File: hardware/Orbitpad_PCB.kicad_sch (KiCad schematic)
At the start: 50 parts, among them J1 Conn_01x04_Pin, SW1 SW_Push, SW10 SW_Push, SW11 SW_Push, SW12 SW_Push, SW13 SW_Push, SW14 SW_Push, SW15 SW_Push, SW16 SW_Push, SW2 SW_Push, SW3 SW_Push, SW4 SW_Push, SW5 SW_Push, SW6 SW_Push, SW7 SW_Push, SW8 SW_Push, SW9 SW_Push, U1 XIAO-RP2040-DIP

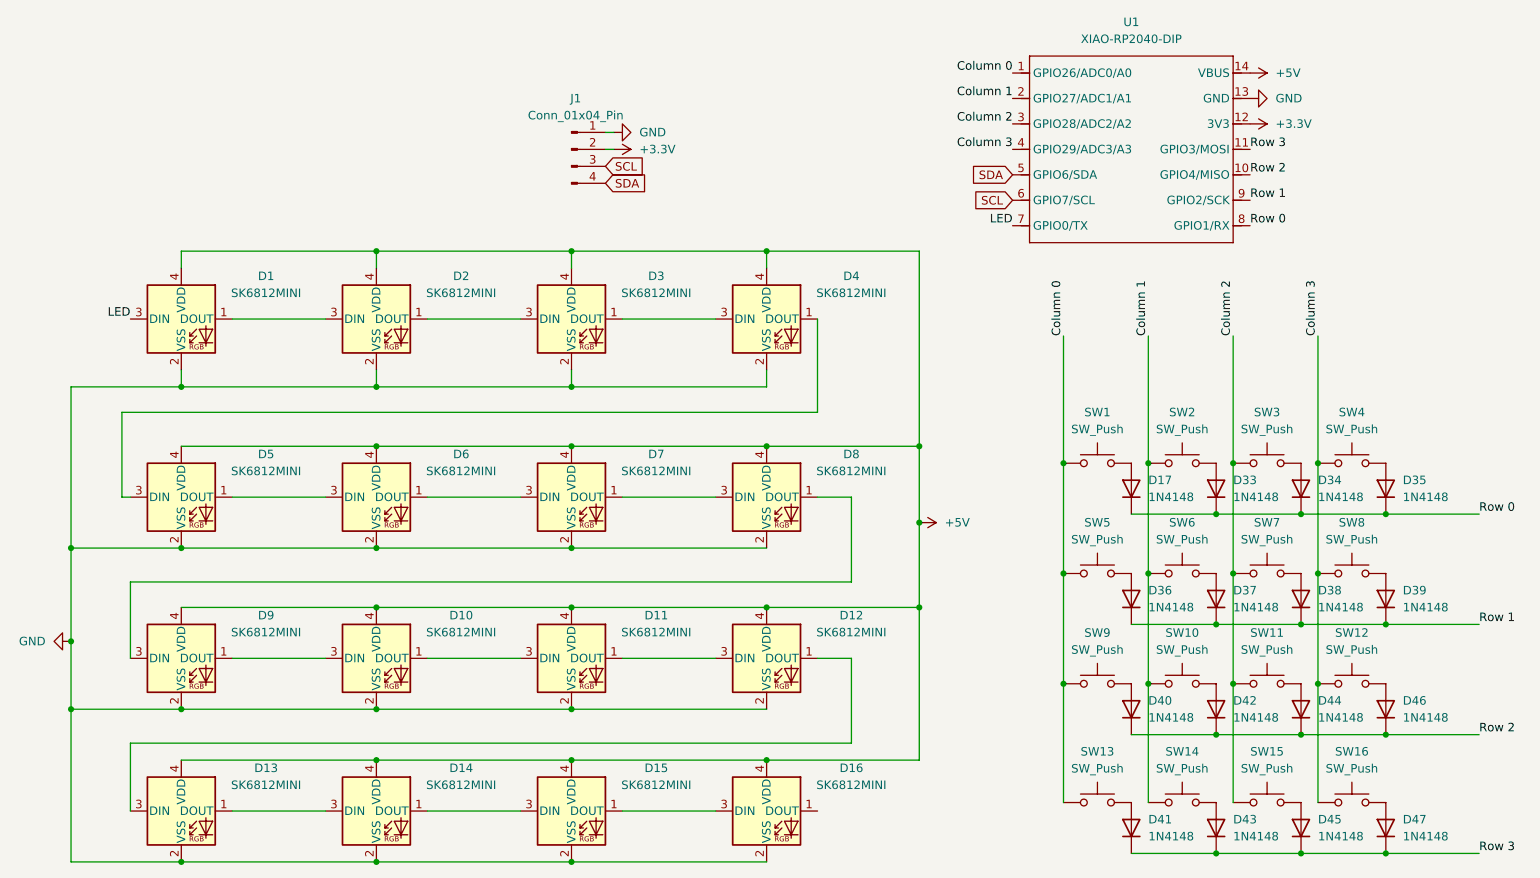
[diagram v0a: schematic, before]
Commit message: Final KiCAD PCB design
These are the final Kicad files for the PCB
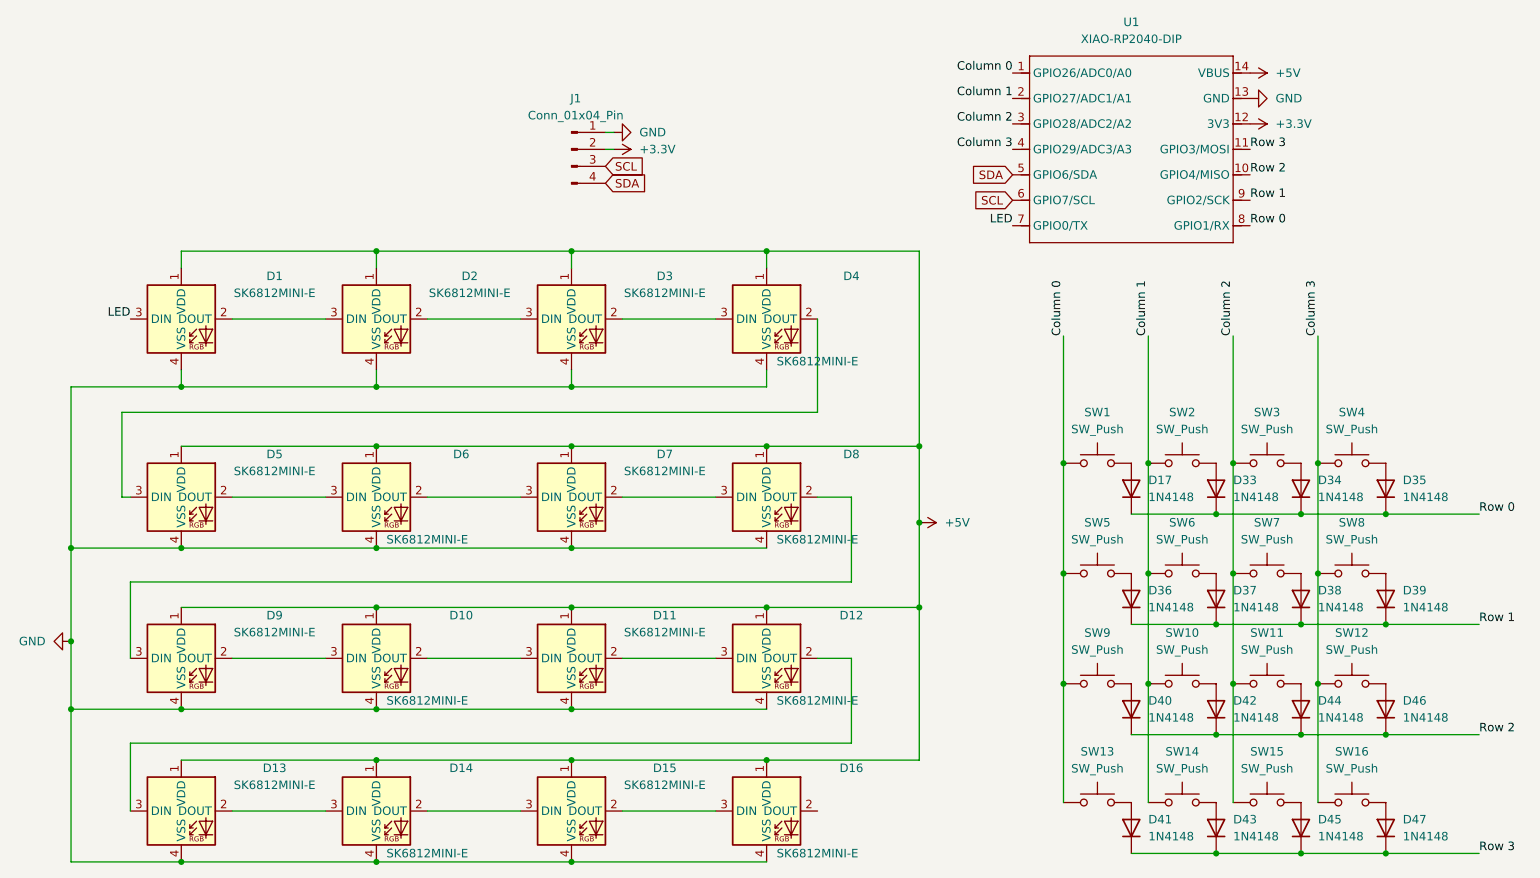
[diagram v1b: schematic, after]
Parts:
- removed D1, D2: SK6812MINI, LED_SMD:LED_SK6812MINI_PLCC4_3.5x3.5mm_P1.75mm, symbol LED:SK6812MINI
- added D1, D2: SK6812MINI-E, PCM_marbastlib-various:LED_6028R, symbol PCM_marbastlib-various:SK6812MINI-E
- D10, D11, D12, D13, D14, D15, D16, D3, D4, D5, D6, D7, D8, D9: value SK6812MINI -> SK6812MINI-E; footprint LED_SMD:LED_SK6812MINI_PLCC4_3.5x3.5mm_P1.75mm -> PCM_marbastlib-various:LED_6028R; symbol LED:SK6812MINI -> PCM_marbastlib-various:SK6812MINI-E
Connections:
- net +5V: now also D10.1 (VDD), D11.1 (VDD), D12.1 (VDD), D13.1 (VDD), D14.1 (VDD), D15.1 (VDD), D16.1 (VDD), D3.1 (VDD), D4.1 (VDD), D5.1 (VDD), D6.1 (VDD), D7.1 (VDD), D8.1 (VDD), D9.1 (VDD), D1.1 (VDD), D2.1 (VDD); no longer D10.4 (VDD), D11.4 (VDD), D12.4 (VDD), D13.4 (VDD), D14.4 (VDD), D15.4 (VDD), D16.4 (VDD), D3.4 (VDD), D4.4 (VDD), D5.4 (VDD), D6.4 (VDD), D7.4 (VDD), D8.4 (VDD), D9.4 (VDD)
- net GND: now also D10.4 (VSS), D11.4 (VSS), D12.4 (VSS), D13.4 (VSS), D14.4 (VSS), D15.4 (VSS), D16.4 (VSS), D3.4 (VSS), D4.4 (VSS), D5.4 (VSS), D6.4 (VSS), D7.4 (VSS), D8.4 (VSS), D9.4 (VSS), D1.4 (VSS), D2.4 (VSS); no longer D10.2 (VSS), D11.2 (VSS), D12.2 (VSS), D13.2 (VSS), D14.2 (VSS), D15.2 (VSS), D16.2 (VSS), D3.2 (VSS), D4.2 (VSS), D5.2 (VSS), D6.2 (VSS), D7.2 (VSS), D8.2 (VSS), D9.2 (VSS)
- net LED: now also D1.3 (DIN)
- net at D6.3 (DIN): now also D5.2 (DOUT); no longer D5.1 (DOUT)
- net at D5.3 (DIN): now also D4.2 (DOUT); no longer D4.1 (DOUT)
- net at D13.3 (DIN): now also D12.2 (DOUT); no longer D12.1 (DOUT)
- net at D12.3 (DIN): now also D11.2 (DOUT); no longer D11.1 (DOUT)
- net at D7.3 (DIN): now also D6.2 (DOUT); no longer D6.1 (DOUT)
- net at D4.3 (DIN): now also D3.2 (DOUT); no longer D3.1 (DOUT)
- net at D3.3 (DIN): now also D2.2 (DOUT)
- net at D11.3 (DIN): now also D10.2 (DOUT); no longer D10.1 (DOUT)
- net at D10.3 (DIN): now also D9.2 (DOUT); no longer D9.1 (DOUT)
- net at D16.3 (DIN): now also D15.2 (DOUT); no longer D15.1 (DOUT)
- net at D15.3 (DIN): now also D14.2 (DOUT); no longer D14.1 (DOUT)
- net at D14.3 (DIN): now also D13.2 (DOUT); no longer D13.1 (DOUT)
- net at D8.3 (DIN): now also D7.2 (DOUT); no longer D7.1 (DOUT)
- net at D9.3 (DIN): now also D8.2 (DOUT); no longer D8.1 (DOUT)
- new net: D1.2 (DOUT), D2.3 (DIN)
